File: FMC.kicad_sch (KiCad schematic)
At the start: 4 parts

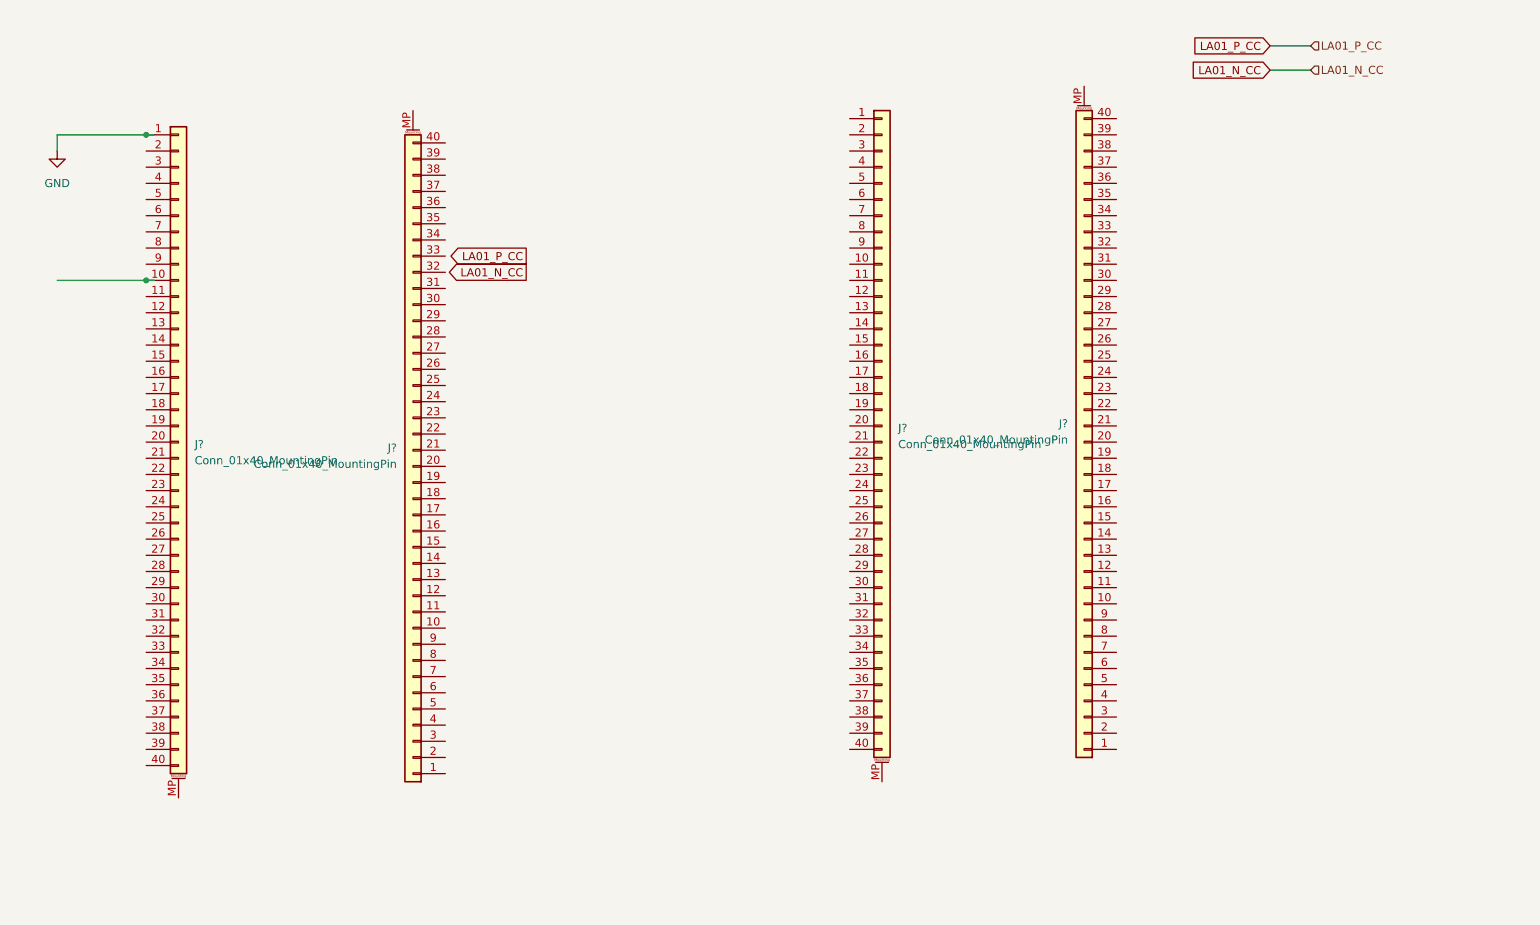
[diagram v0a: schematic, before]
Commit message: Add files via upload
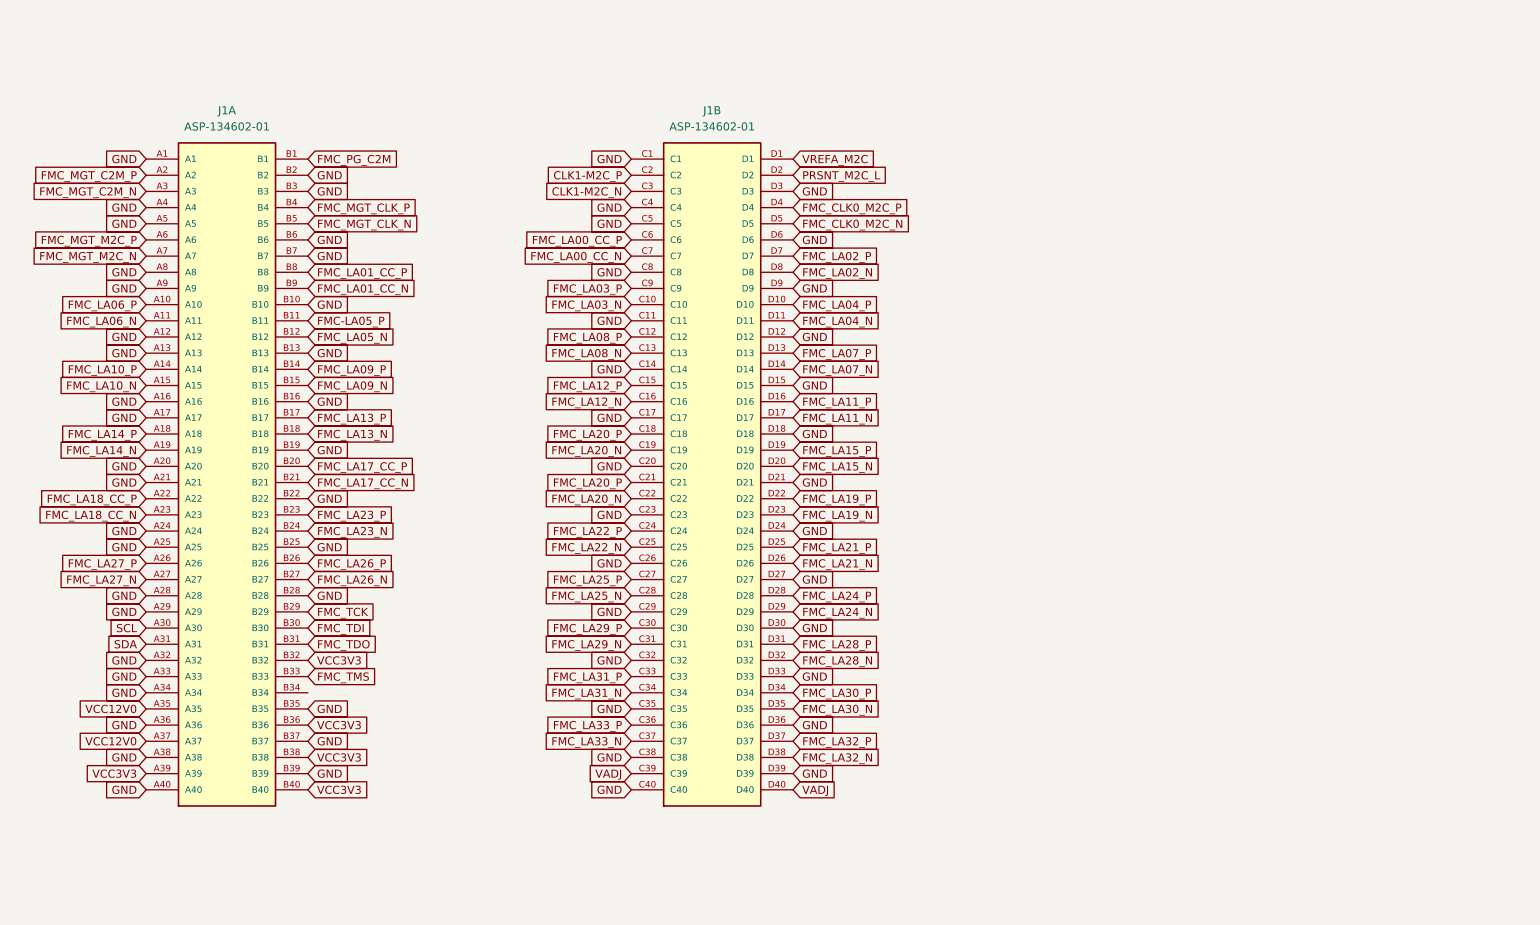
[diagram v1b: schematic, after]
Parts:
- removed J? (x4): Conn_01x40_MountingPin, symbol Connector_Generic_MountingPin:Conn_01x40_MountingPin
- added J1: ASP-134602-01, ASP-134602-01:SAMTEC_ASP-134602-01, symbol ASP-134602-01:ASP-134602-01
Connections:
- net GND: now also J1.A1, J1.A12, J1.A13, J1.A16, J1.A17, J1.A20, J1.A21, J1.A24, J1.A25, J1.A28, J1.A29, J1.A32, J1.A33, J1.A34, J1.A36, J1.A38, J1.A4, J1.A40, J1.A5, J1.A8, J1.A9, J1.B10, J1.B13, J1.B16, J1.B19, J1.B2, J1.B22, J1.B25, J1.B28, J1.B3, J1.B35, J1.B37, J1.B39, J1.B6, J1.B7, J1.C1, J1.C11, J1.C14, J1.C17, J1.C20, J1.C23, J1.C26, J1.C29, J1.C32, J1.C35, J1.C38, J1.C4, J1.C40, J1.C5, J1.C8, J1.D12, J1.D15, J1.D18, J1.D21, J1.D24, J1.D27, J1.D3, J1.D30, J1.D33, J1.D36, J1.D39, J1.D6, J1.D9
- new net CLK1-M2C_N: J1.C3
- new net CLK1-M2C_P: J1.C2
- new net FMC-LA05_P: J1.B11
- new net FMC_CLK0_M2C_N: J1.D5
- new net FMC_CLK0_M2C_P: J1.D4
- new net FMC_LA00_CC_N: J1.C7
- new net FMC_LA00_CC_P: J1.C6
- new net FMC_LA01_CC_N: J1.B9
- new net FMC_LA01_CC_P: J1.B8
- new net FMC_LA02_N: J1.D8
- new net FMC_LA02_P: J1.D7
- new net FMC_LA03_N: J1.C10
- new net FMC_LA03_P: J1.C9
- new net FMC_LA04_N: J1.D11
- new net FMC_LA04_P: J1.D10
- new net FMC_LA05_N: J1.B12
- new net FMC_LA06_N: J1.A11
- new net FMC_LA06_P: J1.A10
- new net FMC_LA07_N: J1.D14
- new net FMC_LA07_P: J1.D13
- new net FMC_LA08_N: J1.C13
- new net FMC_LA08_P: J1.C12
- new net FMC_LA09_N: J1.B15
- new net FMC_LA09_P: J1.B14
- new net FMC_LA10_N: J1.A15
- new net FMC_LA10_P: J1.A14
- new net FMC_LA11_N: J1.D17
- new net FMC_LA11_P: J1.D16
- new net FMC_LA12_N: J1.C16
- new net FMC_LA12_P: J1.C15
- new net FMC_LA13_N: J1.B18
- new net FMC_LA13_P: J1.B17
- new net FMC_LA14_N: J1.A19
- new net FMC_LA14_P: J1.A18
- new net FMC_LA15_N: J1.D20
- new net FMC_LA15_P: J1.D19
- new net FMC_LA17_CC_N: J1.B21
- new net FMC_LA17_CC_P: J1.B20
- new net FMC_LA18_CC_N: J1.A23
- new net FMC_LA18_CC_P: J1.A22
- new net FMC_LA19_N: J1.D23
- new net FMC_LA19_P: J1.D22
- new net FMC_LA20_N: J1.C19, J1.C22
- new net FMC_LA20_P: J1.C18, J1.C21
- new net FMC_LA21_N: J1.D26
- new net FMC_LA21_P: J1.D25
- new net FMC_LA22_N: J1.C25
- new net FMC_LA22_P: J1.C24
- new net FMC_LA23_N: J1.B24
- new net FMC_LA23_P: J1.B23
- new net FMC_LA24_N: J1.D29
- new net FMC_LA24_P: J1.D28
- new net FMC_LA25_N: J1.C28
- new net FMC_LA25_P: J1.C27
- new net FMC_LA26_N: J1.B27
- new net FMC_LA26_P: J1.B26
- new net FMC_LA27_N: J1.A27
- new net FMC_LA27_P: J1.A26
- new net FMC_LA28_N: J1.D32
- new net FMC_LA28_P: J1.D31
- new net FMC_LA29_N: J1.C31
- new net FMC_LA29_P: J1.C30
- new net FMC_LA30_N: J1.D35
- new net FMC_LA30_P: J1.D34
- new net FMC_LA31_N: J1.C34
- new net FMC_LA31_P: J1.C33
- new net FMC_LA32_N: J1.D38
- new net FMC_LA32_P: J1.D37
- new net FMC_LA33_N: J1.C37
- new net FMC_LA33_P: J1.C36
- new net FMC_MGT_C2M_N: J1.A3
- new net FMC_MGT_C2M_P: J1.A2
- new net FMC_MGT_CLK_N: J1.B5
- new net FMC_MGT_CLK_P: J1.B4
- new net FMC_MGT_M2C_N: J1.A7
- new net FMC_MGT_M2C_P: J1.A6
- new net FMC_PG_C2M: J1.B1
- new net FMC_TCK: J1.B29
- new net FMC_TDI: J1.B30
- new net FMC_TDO: J1.B31
- new net FMC_TMS: J1.B33
- new net PRSNT_M2C_L: J1.D2
- new net SCL: J1.A30
- new net SDA: J1.A31
- new net VADJ: J1.C39, J1.D40
- new net VCC12V0: J1.A35, J1.A37
- new net VCC3V3: J1.A39, J1.B32, J1.B36, J1.B38, J1.B40
- new net VREFA_M2C: J1.D1

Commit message: Add files via upload
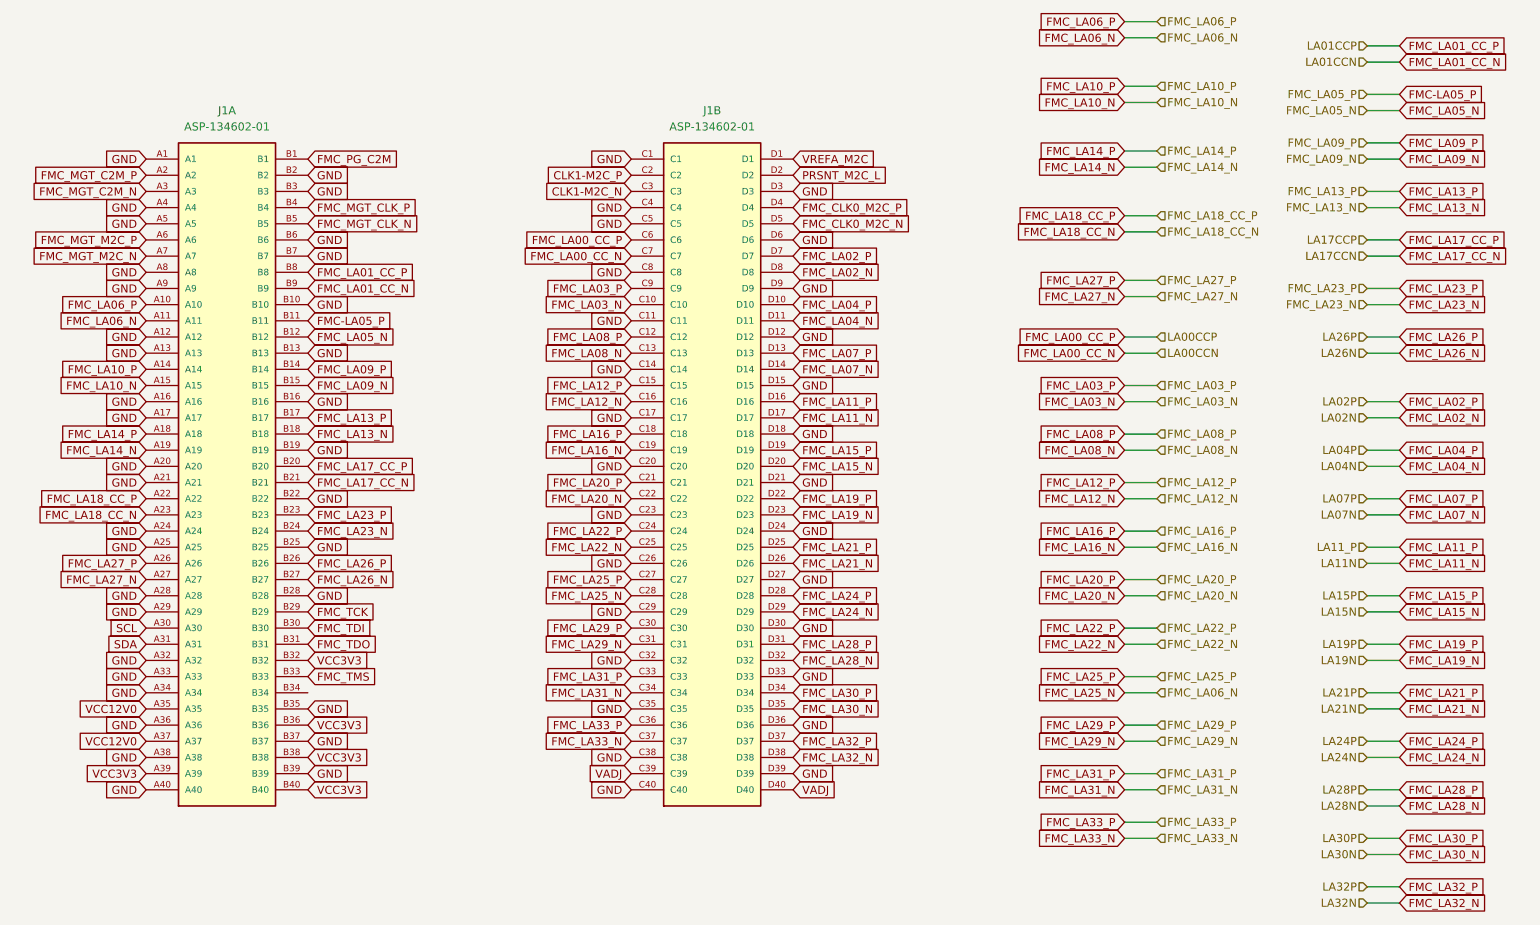
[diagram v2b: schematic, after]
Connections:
- net FMC_LA25_N is gone; now on net FMC_LA06_N: J1.C28
- net FMC_LA20_N: no longer J1.C19
- net FMC_LA20_P: no longer J1.C18
- new net FMC_LA16_N: J1.C19
- new net FMC_LA16_P: J1.C18

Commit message: Add files via upload
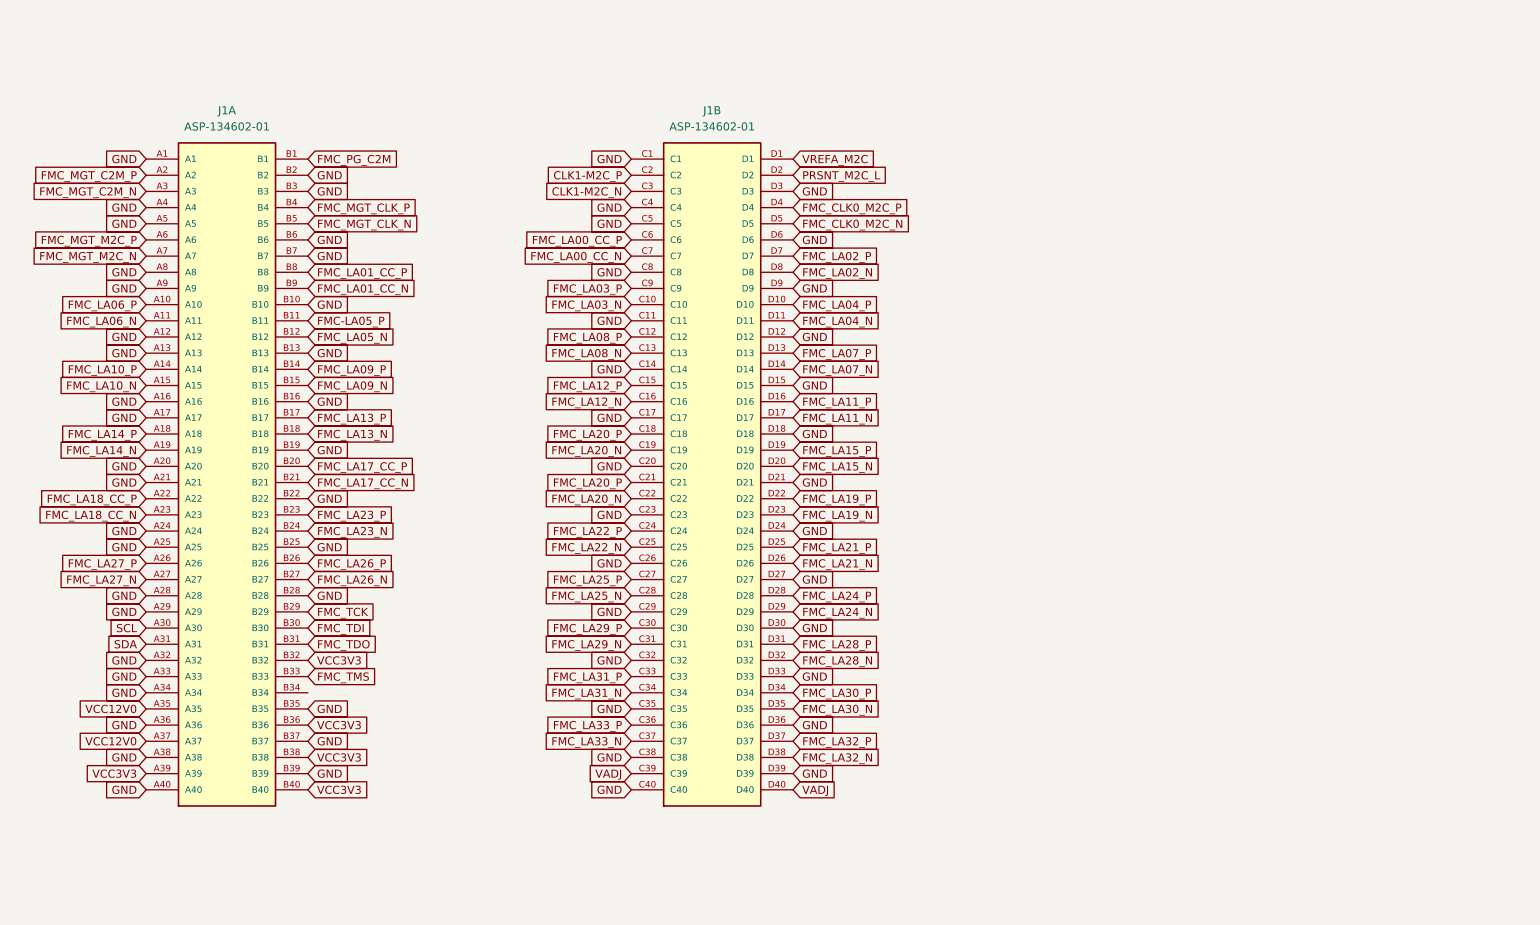
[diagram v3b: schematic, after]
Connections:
- net FMC_LA16_N is gone; now on net FMC_LA20_N: J1.C19
- net FMC_LA16_P is gone; now on net FMC_LA20_P: J1.C18
- net FMC_LA06_N: no longer J1.C28
- new net FMC_LA25_N: J1.C28
